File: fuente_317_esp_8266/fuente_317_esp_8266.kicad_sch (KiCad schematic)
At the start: 35 parts, among them J1 UART, J10 Alimentacion, J12 Vadj+, J13 Vadj-, J2 LCD16x2, J3 Vadj+, J4 Vadj-, J5 Vadj+, J6 Vadj-, J8 BTN_MODE, J9 BTN_SEL, U2 CD4051B, U3 LM324, U4 AMS1117-3.3

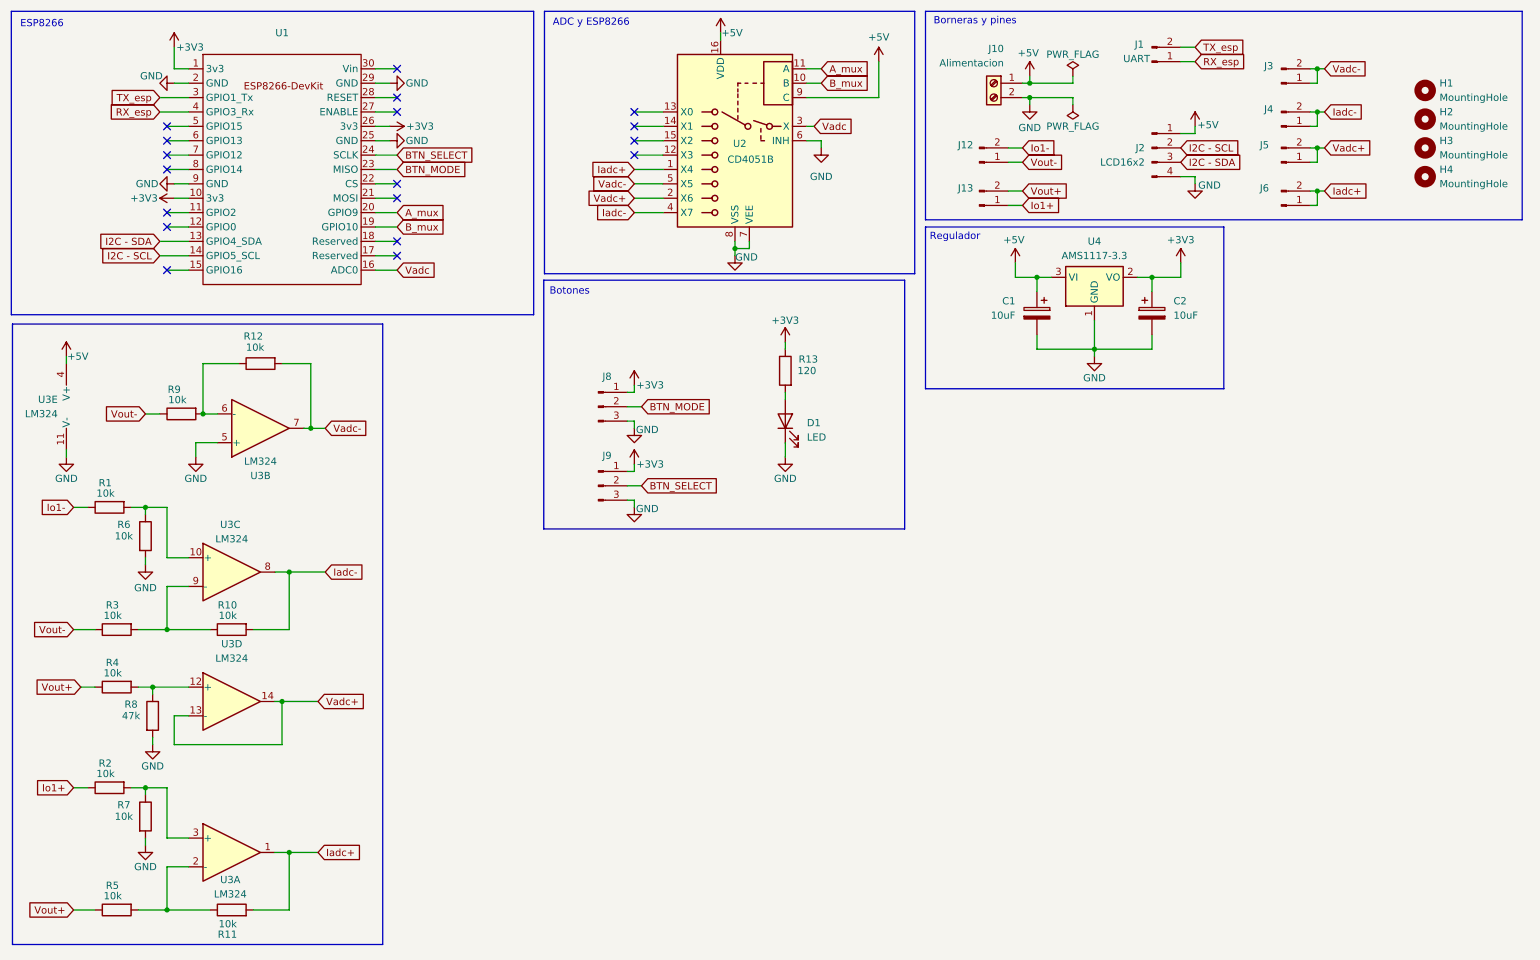
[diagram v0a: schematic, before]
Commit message: feat: version final para el tp integrador
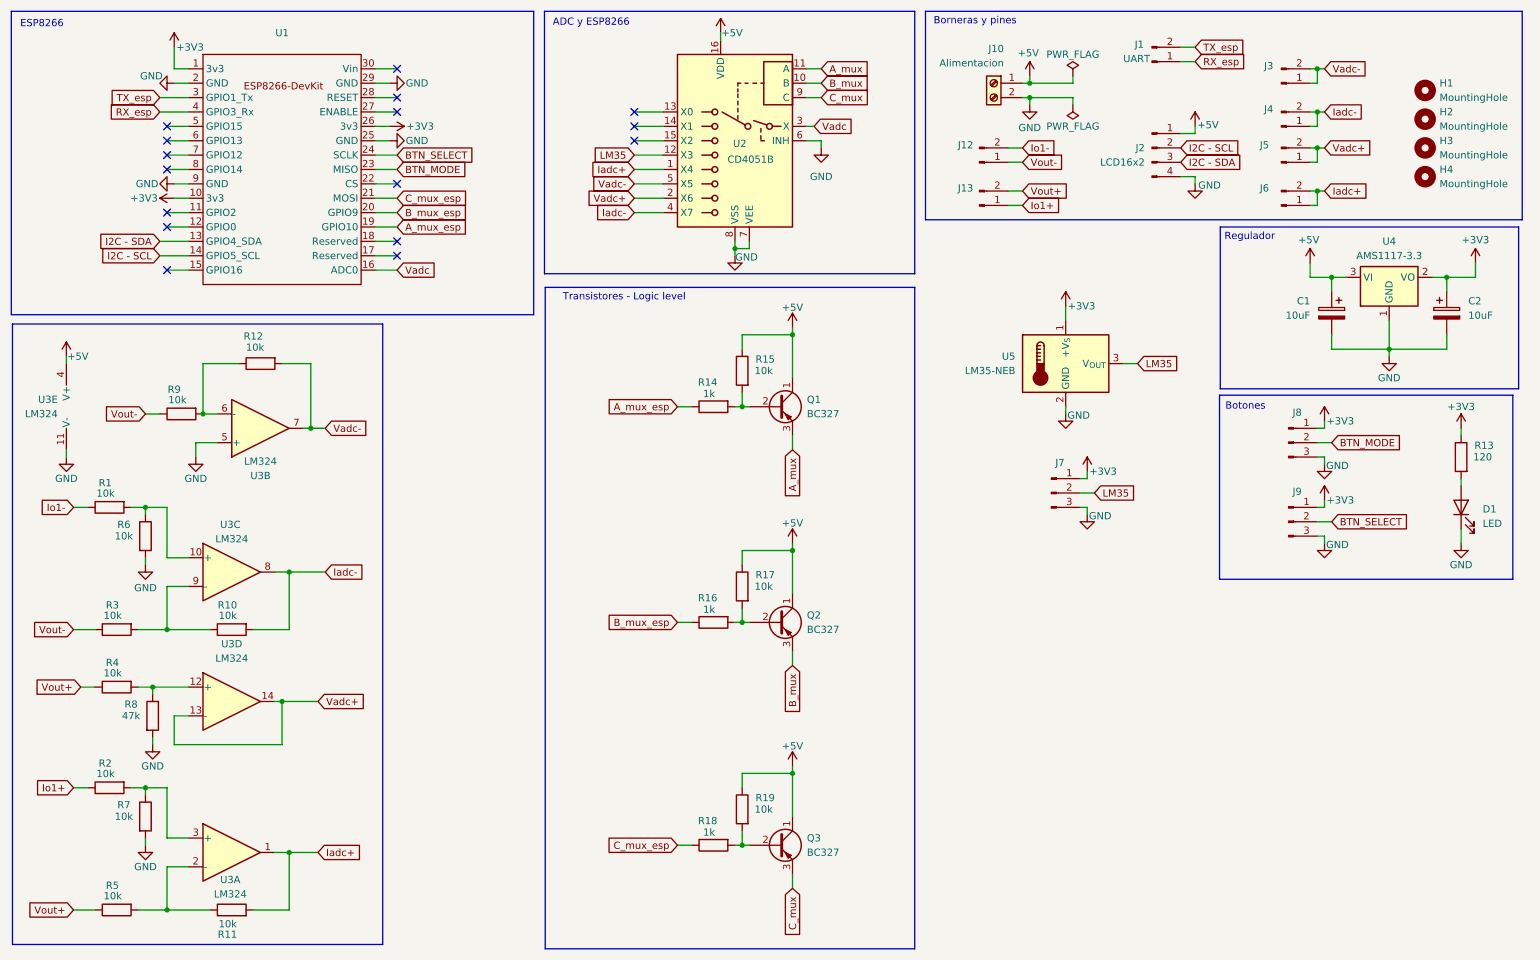
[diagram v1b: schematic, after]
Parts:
- added J7: BTN_SEL, Connector_PinHeader_2.54mm:PinHeader_1x03_P2.54mm_Vertical, symbol Connector:Conn_01x03_Pin
- added Q1, Q2, Q3: BC327, Package_TO_SOT_THT:TO-92_Inline, symbol Transistor_BJT:BC327
- added R14, R16, R18: 1k, Resistor_THT:R_Axial_DIN0207_L6.3mm_D2.5mm_P10.16mm_Horizontal, symbol Device:R
- added R15, R17, R19: 10k, Resistor_THT:R_Axial_DIN0207_L6.3mm_D2.5mm_P10.16mm_Horizontal, symbol Device:R
- added U5: LM35-NEB, Package_TO_SOT_THT:TO-220-3_Vertical, symbol Sensor_Temperature:LM35-NEB
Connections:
- net +3V3: now also J7.1 (Pin_1), U5.1 (+V_{S})
- net +5V: now also Q1.1 (C), Q2.1 (C), Q3.1 (C), R15.1, R17.1, R19.1; no longer U2.9 (C)
- net A_mux: now also Q1.3 (E); no longer U1.20 (GPIO9)
- net B_mux: now also Q2.3 (E); no longer U1.19 (GPIO10)
- net GND: now also J7.3 (Pin_3), U5.2 (GND)
- net C_mux_esp: now reaches U1.21 (MOSI)
- net C_mux_esp: now also R18.1
- net LM35: now reaches U2.12 (X3)
- net LM35: now also J7.2 (Pin_2), U5.3 (V_{OUT})
- new net: Q1.2 (B), R14.2, R15.2
- new net: Q2.2 (B), R16.2, R17.2
- new net: Q3.2 (B), R18.2, R19.2
- new net A_mux_esp: R14.1, U1.19 (GPIO10)
- new net B_mux_esp: R16.1, U1.20 (GPIO9)
- new net C_mux: Q3.3 (E), U2.9 (C)
- no-connect marks 18 -> 16
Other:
- note added: "Transistores - Logic level"
- moved on the sheet: C1, C2, D1, J8, J9, R13, U4
